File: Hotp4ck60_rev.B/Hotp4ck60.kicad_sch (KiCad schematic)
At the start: 41 parts, among them J1 JST, SW44 Reset, U1 nRF52840, Y1 32 MHz, Y2 32.768 Khz

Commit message: Change to daugtherboard
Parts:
- removed AE1: 2.4 GHz ANT, RF_Antenna:Texas_SWRA117D_2.4GHz_Right, symbol Device:Antenna_Dipole
- removed C15, C19, C20: 4.7 uF, Capacitor_SMD:C_0402_1005Metric, symbol Device:C_Small
- removed C16, C17, C18: 100 nF, Capacitor_SMD:C_0402_1005Metric, symbol Device:C_Small
- removed C4, C5: 12 pF, Capacitor_SMD:C_0402_1005Metric, symbol Device:C
- removed L1: 4.7 nH, Inductor_SMD:L_0402_1005Metric, symbol Device:L_Small
- removed L3: 15 nH, Inductor_SMD:L_0402_1005Metric, symbol Device:L_Small
- removed L4: 10 uH, Inductor_SMD:L_0603_1608Metric, symbol Device:L_Small
- removed LED1: Blue, LED_SMD:LED_0603_1608Metric, symbol Device:LED_Small
- removed SW44: Reset, marbastlib-various:SW_SPST_SKQG_WithStem, symbol Switch:SW_SPST
- removed U1: nRF52840, Package_DFN_QFN:Nordic_AQFN-73-1EP_7x7mm_P0.5mm, symbol MCU_Nordic:nRF52840
- removed Y1: 32 MHz, Crystal:Crystal_SMD_2016-4Pin_2.0x1.6mm, symbol Device:Crystal_GND24_Small
- removed Y2: 32.768 Khz, Crystal:Crystal_SMD_2012-2Pin_2.0x1.2mm, symbol Device:Crystal
- added C6: 100n, Capacitor_SMD:C_0402_1005Metric, symbol Device:C_Small
- added C7: 4u7, Capacitor_SMD:C_0402_1005Metric, symbol Device:C_Small
- added J2: Conn_01x02_MountingPin, Connector_Molex:Molex_PicoBlade_53261-0271_1x02-1MP_P1.25mm_Horizontal, symbol Connector_Generic_MountingPin:Conn_01x02_MountingPin
- added LED1: IND, PCM_marbastlib-various:LED_1206R, symbol PCM_marbastlib-various:LED_MHT151RGBCT
- added PWR1: PWR, PCM_marbastlib-various:SW_MSK12C02-HB, symbol Switch:SW_Push_SPDT
- added Q1: 2N7002, Package_TO_SOT_SMD:SOT-23, symbol Transistor_FET:2N7002
- added R10, R11, R9: 1k, Resistor_SMD:R_0402_1005Metric, symbol Device:R_Small
- added R12: 100 Ohm, Resistor_SMD:R_0402_1005Metric, symbol Device:R_Small
- added R13: 10 kOhm, Resistor_SMD:R_0402_1005Metric, symbol Device:R_Small
- added R14: 100 kOhm, Resistor_SMD:R_0402_1005Metric, symbol Device:R_Small
- added R4: 47k, Resistor_SMD:R_0402_1005Metric, symbol Device:R_Small
- added R5: 1k5, Resistor_SMD:R_0402_1005Metric, symbol Device:R_Small
- added R6: 2k2, Resistor_SMD:R_0402_1005Metric, symbol Device:R_Small
- added R7, R8: 10k, Resistor_SMD:R_0402_1005Metric, symbol Device:R_Small
- added RST1: RST, PCM_marbastlib-various:SW_T1A2QR, symbol Switch:SW_Push
- added U1: MAX17048, Package_DFN_QFN:DFN-8-1EP_2x2mm_P0.5mm_EP0.6x1.2mm, symbol marbastlib-various:MAX17048
- added U2: BQ24075, Package_DFN_QFN:VQFN-16-1EP_3x3mm_P0.5mm_EP1.6x1.6mm, symbol Battery_Management:BQ24075RGT
- added U3: nRF52840_E73-2G4M08S1C, PCM_marbastlib-various:nRF52840_E73-2G4M08S1C, symbol PCM_marbastlib-various:nRF52840_E73-2G4M08S1C
- added U5: 74LVC1G11, Package_TO_SOT_SMD:SOT-363_SC-70-6, symbol 74xGxx:74LVC1G11
- added Y1: 32.768 KHz, Crystal:Crystal_SMD_2012-2Pin_2.0x1.2mm, symbol Device:Crystal_Small
- C1, C2: value 12 pF -> 4u7; LCSC C1547 -> C23733; Notes NP0, 2% -> X7R, 10%
- C10: value 4.7 uF -> 4u7
- C11: value 820 pF -> 4u7; LCSC C161159 -> C23733; Notes NP0, 5% -> X7R, 10%
- C12: value 100 pF -> 12p; LCSC C1546 -> C1547; Notes NP0, 5% -> NP0, 2%
- C13: value 100 nF -> 12p; LCSC C1525 -> C1547; Notes X7R, 10% -> NP0, 2%
- C14: value 1 uF -> 100n; LCSC C52923 -> C307331; Notes X7R, 10% -> (none)
- C3: value NC -> 1u; LCSC C77179 -> C52923; Notes (none) -> X7R, 10%; now in the parts list
- C4: value 0.5 pF -> 4u7; LCSC C77179 -> C23733; Notes NP0, 10% -> X7R, 10%
- C5: value 0.8 pF -> 1u; LCSC C285068 -> C52923; Notes NP0, 10% -> X7R, 10%
- C8: value 1 uF -> 1u
- C9: value 47 nF -> 1u; footprint Capacitor_SMD:C_0603_1608Metric -> Capacitor_SMD:C_0402_1005Metric; LCSC C26403 -> C52923
- L2: LCSC C252081 -> C92982; Notes 50 mA, 20% -> 80 mA, 20%
- R3: value 1 kOhm -> 10k; LCSC C25890 -> C25744
- renumbered H2 to H?, H4 to H?, H1 to H?, H3 to H?, H5 to H?, H6 to H?, H7 to H?
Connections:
- net DCC is gone; now on net DCCH: L2.1
- net DEC5 is gone; now on net +VSW: C11.1
- net +5V: now also C1.1, C10.1, C2.1, C3.1, R12.1, U2.13 (IN), U3.27 (VBUS)
- net +VSW: now also C4.1, C5.1, U2.10 (OUT), U2.11 (OUT), U2.6 (EN1), U3.23 (VDDH); no longer C10.1
- net D+: now also U3.31 (D+)
- net D-: now also U3.29 (D-)
- net DCCH: now also U3.25 (DCCH)
- net GND: now also C3.2, C4.2, C5.2, R3.2, C6.2, C7.2, J2.2 (Pin_2), J2.MP (MountPin), PWR1.3 (C), Q1.2 (S), R13.2, R4.2, R5.2, R6.2, RST1.2, U1.1 (CTG), U1.4 (GND), U1.6 (QSTRT), U1.9 (GND), U2.17 (VSS), U2.4 (~{CE}), U2.5 (EN2), U2.8 (VSS), U3.21 (GND), U3.24 (GND), U3.5 (GND), U5.2 (GND); no longer C3.1, C4.1, C5.1
- net RST: now also RST1.1, U3.26 (P0.18/~{RESET})
- net SCL: now also R8.2, U1.7 (SCL), U3.17 (P1.09)
- net SDA: now also R7.2, U1.8 (SDA), U3.15 (P0.05/AIN3)
- net SWDCLK: now also U3.39 (SWDCLK)
- net SWDIO: now also U3.37 (SWDIO)
- net VDD: now also C9.1, L2.2, LED1.1 (A), R7.1, R8.1, U3.19 (VDD), U5.5 (VCC)
- net DEC1: no longer names the net of C13.1
- net DEC1: now also U3.13 (P0.01/XL2), Y1.1
- net DEC3: no longer names the net of C12.1
- net DEC3: now also U3.11 (P0.00/XL1), Y1.2
- net DEC4_6 renamed +BATT
- net +BATT: now also C6.1, C7.1, J2.1 (Pin_1), R14.2, U1.2 (CELL), U1.3 (VDD), U2.2 (BAT), U2.3 (BAT); no longer C9.1
- net LED: no longer names the net of R3.1
- net LED: now also U2.1 (TS)
- new net: R6.1, U2.16 (ISET)
- new net: Q1.1 (G), R12.2, R13.1
- new net: LED1.3 (GK), R10.1
- new net: PWR1.1 (A), R14.1
- new net: LED1.2 (BK), R9.1
- new net: LED1.4 (RK), R11.1
- new net ALERT: U1.5 (~{ALRT})
- new net ILIM: R5.1, U2.12 (ILIM)
- new net LED_B: R9.2, U3.38 (P1.02)
- new net LED_G: R10.2, U3.36 (P1.00)
- new net SYSOFF: PWR1.2 (B), Q1.3 (D), U2.15 (SYSOFF)
- new net TMR: R4.1, U2.14 (TMR)
- new net c00: U3.41 (P0.09/NFC1)
- new net c01: U3.34 (P0.22)
- new net c02: U3.43 (P0.10/NFC2)
- new net c03: U3.28 (P0.15)
- new net c04: U3.32 (P0.20)
- new net c05: U3.33 (P0.13)
- new net c06: U3.3 (P0.03/AIN1)
- new net c07: U3.4 (P0.28/AIN4)
- new net c08: U3.7 (P0.02/AIN0)
- new net c09: U3.8 (P0.29/AIN5)
- new net c10: U3.9 (P0.31/AIN7)
- new net c11: U3.10 (P0.30/AIN6)
- new net r0: U3.12 (P0.26)
- new net r1: U3.14 (P0.06)
- new net r2: U3.16 (P0.08)
- new net r3: U3.30 (P0.17)
- new net wk: U3.22 (P0.07), U5.4
- new net wk1: U5.6
- new net wk2: U5.3
- new net wk3: U5.1
- new net ~{CHG}: R11.2, U2.9 (~{CHG})
- no-connect marks 21 -> 8
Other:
- removed sheet Battery
- note added: "AND gate for ZMK soft poweroff feature"
- note added: "Battery management"
- note added: "Blue and Green connected to MCU GPIOs Red connected to charger output"
- note added: "External DCCH inductor for DC-DC HV input mode"
- note added: "External LF crystal for lower idle power"
- note added: "Fuel Gauge"
- note added: "Indicator LED"
- note added: "Pull-ups for i2c"
- note added: "SYSOFF 1 (SW1 pos 1): Batt OFF SYSOFF 0 (SW1 pos 3): Batt ON"
- note added: "TMR: (10 x 48 s/kOhm) * 47 kOhm = 22560s = 6.27h ILIM: 1550 AOhm / 1500 Ohm = 1.03 A = 1030 mA ISET: 890 AOhm / 2200 Ohm = 0.404 A = 440 mA EN1: 1, EN2: 0 = 475 mA MAX TS: 10 kOhm to GND = no OTP"
- note added: "USB Port"
- note added: "nRF52 module with peripherals"
- moved on the sheet: H?

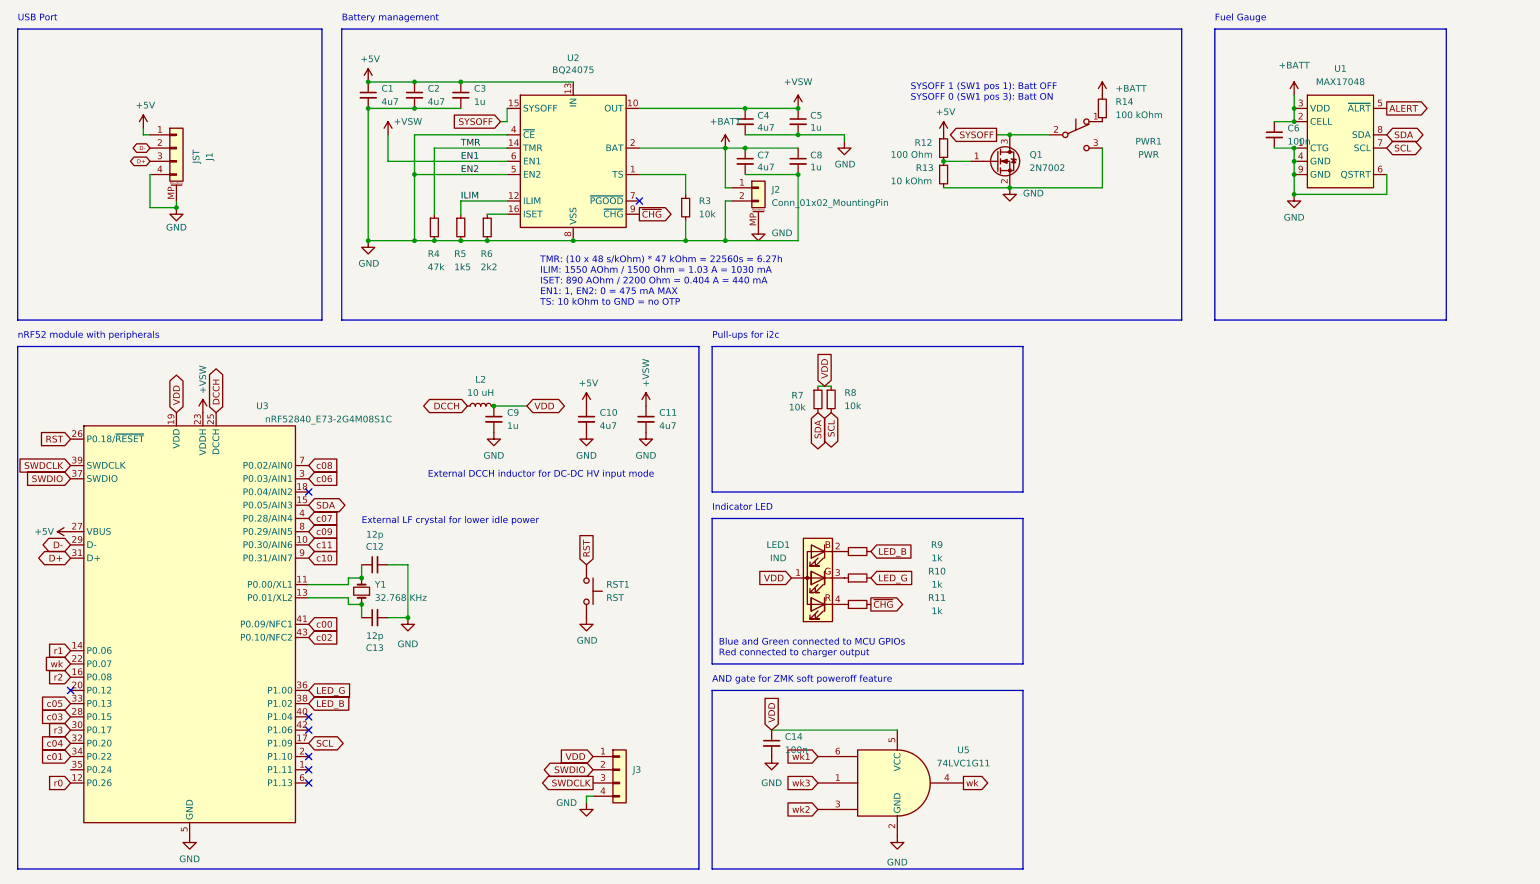
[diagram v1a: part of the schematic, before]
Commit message: place parts and trace connect
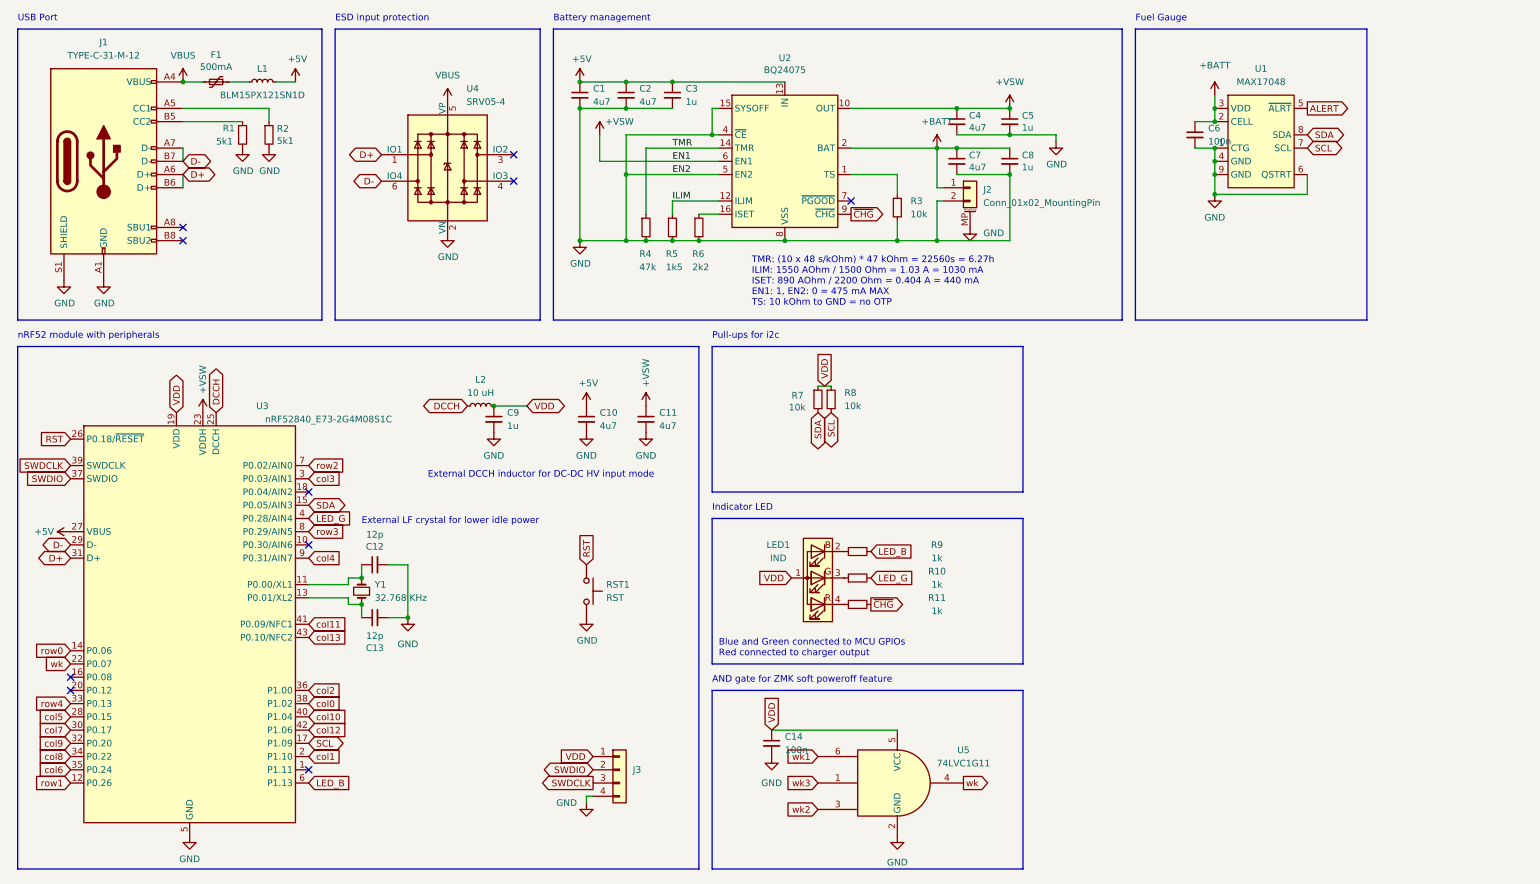
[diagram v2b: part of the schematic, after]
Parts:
- removed J1: JST, Connector_JST:JST_SH_SM04B-SRSS-TB_1x04-1MP_P1.00mm_Horizontal, symbol Connector_Generic_MountingPin:Conn_01x04_MountingPin
- removed PWR1: PWR, PCM_marbastlib-various:SW_MSK12C02-HB, symbol Switch:SW_Push_SPDT
- removed Q1: 2N7002, Package_TO_SOT_SMD:SOT-23, symbol Transistor_FET:2N7002
- removed R12: 100 Ohm, Resistor_SMD:R_0402_1005Metric, symbol Device:R_Small
- removed R13: 10 kOhm, Resistor_SMD:R_0402_1005Metric, symbol Device:R_Small
- removed R14: 100 kOhm, Resistor_SMD:R_0402_1005Metric, symbol Device:R_Small
- added F1: 500mA, Fuse:Fuse_0603_1608Metric, symbol Device:Polyfuse_Small
- added J1: TYPE-C-31-M-12, PCM_marbastlib-various:USB_C_Receptacle_HRO_TYPE-C-31-M-12, symbol Connector:USB_C_Receptacle_USB2.0
- added L1: BLM15PX121SN1D, Inductor_SMD:L_0402_1005Metric, symbol Device:L_Small
- added R1, R2: 5k1, Resistor_SMD:R_0402_1005Metric, symbol Device:R_Small
- added U4: SRV05-4, PCM_marbastlib-various:SOT-23-6-routable, symbol PCM_marbastlib-various:SRV05-4
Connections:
- net SYSOFF is gone; now on net GND: U2.15 (SYSOFF)
- net c07 is gone; now on net LED_G: U3.4 (P0.28/AIN4)
- net +5V: now also L1.2
- net D+: now also J1.A6 (D+), J1.B6 (D+), U4.1 (IO1)
- net D-: now also J1.A7 (D-), J1.B7 (D-), U4.6 (IO4)
- net GND: now also J1.A1 (GND), J1.A12 (GND), J1.B1 (GND), J1.B12 (GND), J1.S1 (SHIELD), R1.2, R2.2, U4.2 (VN)
- net LED_B: now also U3.6 (P1.13); no longer U3.38 (P1.02)
- net LED_G: no longer U3.36 (P1.00)
- net col1: now reaches U3.2 (P1.10)
- net col6: now reaches U3.35 (P0.24)
- net col10: now reaches U3.40 (P1.04)
- net col12: now reaches U3.42 (P1.06)
- net c00 renamed col11
- net c01 renamed col8
- net c02 renamed col13
- net c03 renamed col5
- net c04 renamed col9
- net c05 renamed row4
- net c06 renamed col3
- net c08 renamed row2
- net c09 renamed row3
- net c10 renamed col4
- net c11: no longer names the net of U3.10 (P0.30/AIN6)
- net r0 renamed row1
- net r1 renamed row0
- net r2: no longer names the net of U3.16 (P0.08)
- net r3 renamed col7
- new net: J1.A5 (CC1), R2.1
- new net: J1.B5 (CC2), R1.1
- new net: F1.1, L1.1
- new net VBUS: F1.2, J1.A4 (VBUS), J1.A9 (VBUS), J1.B4 (VBUS), J1.B9 (VBUS), U4.5 (VP)
- new net col0: U3.38 (P1.02)
- new net col2: U3.36 (P1.00)
- no-connect marks 8 -> 10
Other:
- note added: "ESD input protection"
- note removed: "SYSOFF 1 (SW1 pos 1): Batt OFF SYSOFF 0 (SW1 pos 3): Batt ON"
- moved on the sheet: C1, C2, C3, C4, C5, C6, C7, C8, J2, R3, R4, R5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
